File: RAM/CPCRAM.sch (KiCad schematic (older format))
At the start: 11 parts, among them J1 Conn_01x16_Female

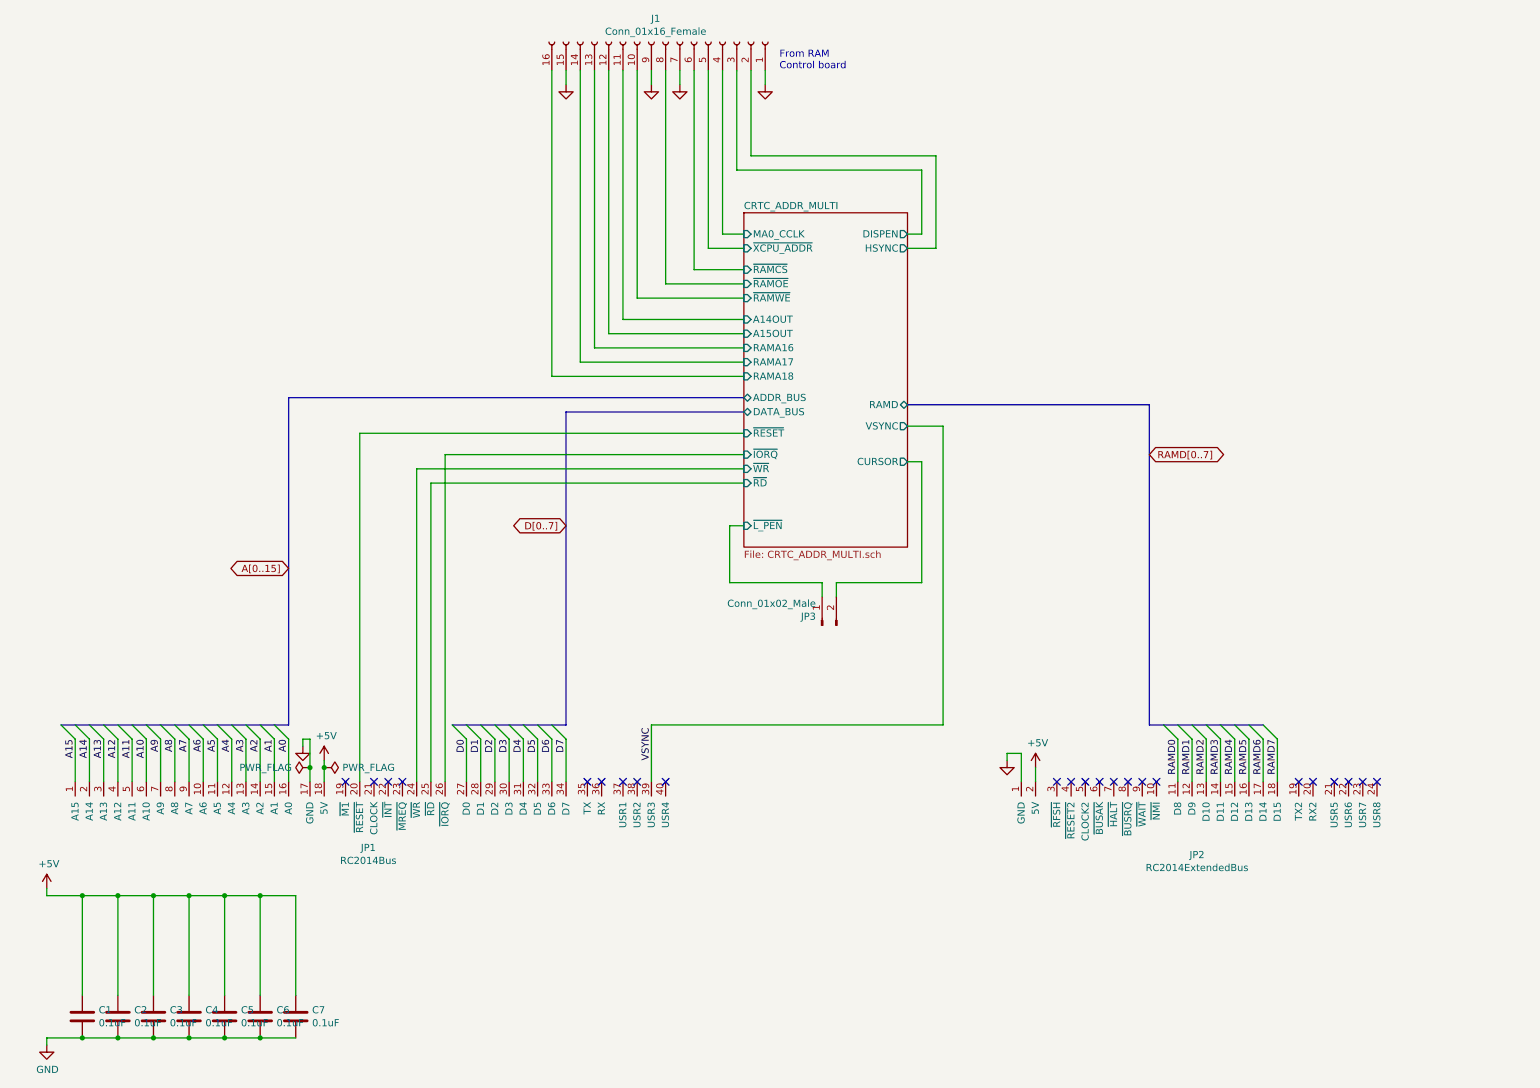
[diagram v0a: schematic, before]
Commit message: Long overdue update...
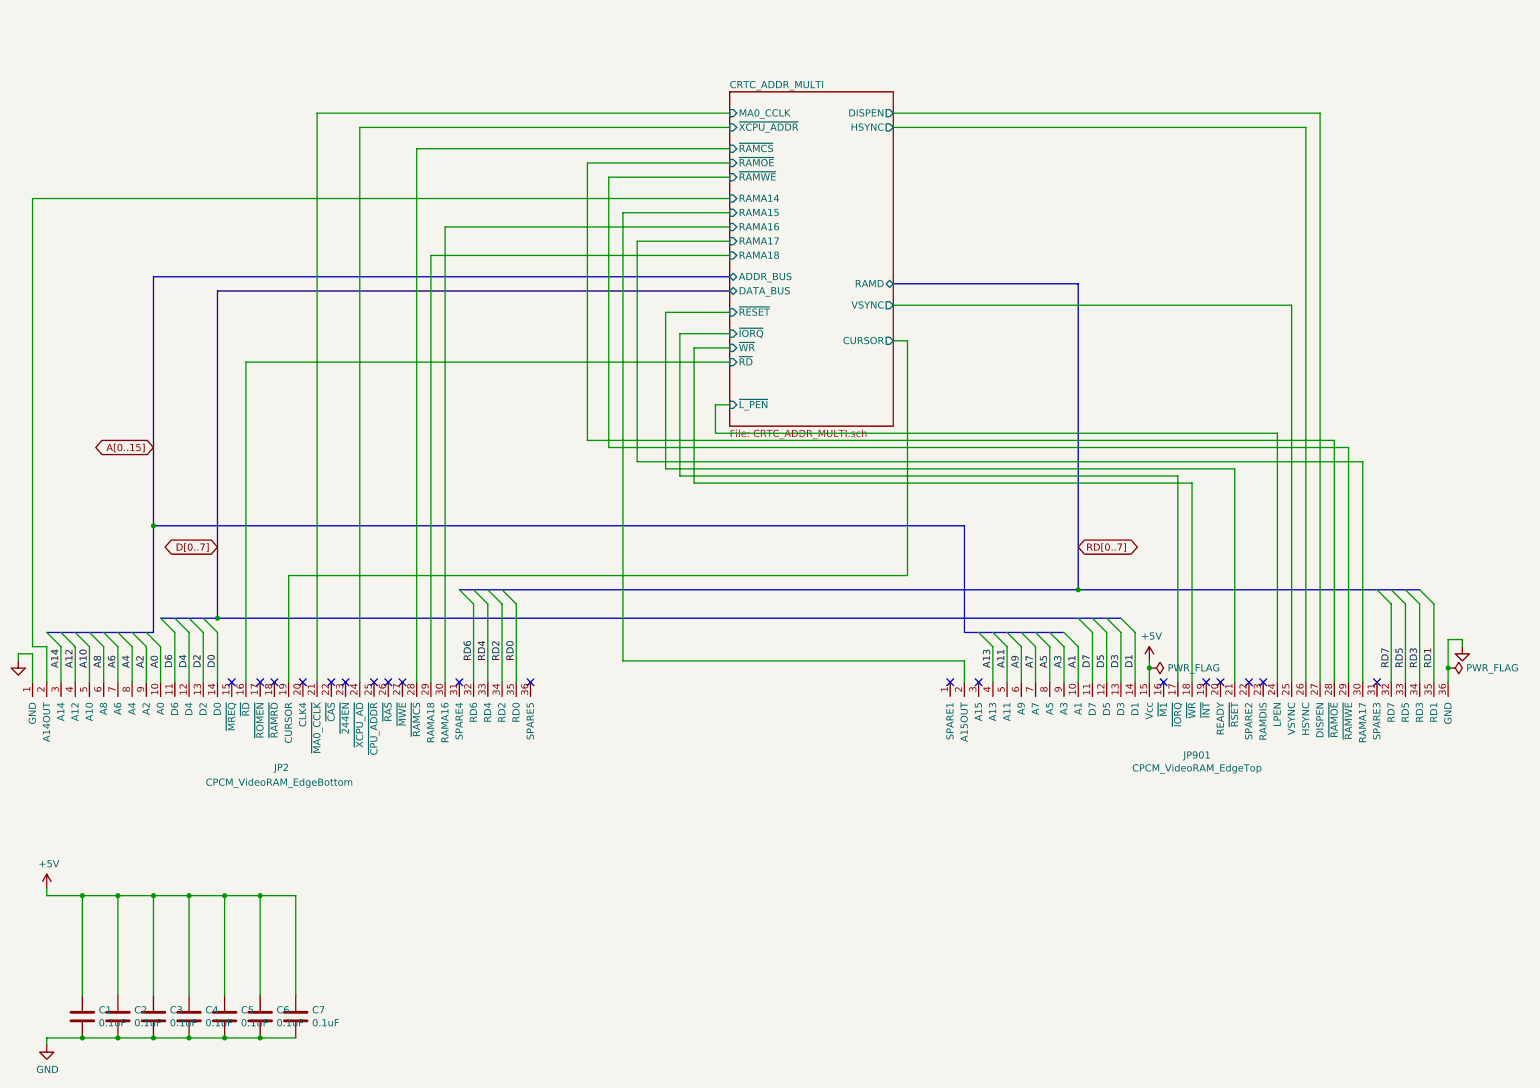
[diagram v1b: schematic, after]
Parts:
- removed J1: Conn_01x16_Female, Connector_PinSocket_2.54mm:PinSocket_2x08_P2.54mm_Vertical, symbol Connector:Conn_01x16_Female
- removed JP1: RC2014Bus, Connector_PinHeader_2.54mm:PinHeader_1x40_P2.54mm_Vertical, symbol CPCRAM-rescue:RC2014Bus-CPC
- removed JP2: RC2014ExtendedBus, Connector_PinHeader_2.54mm:PinHeader_1x25_P2.54mm_Vertical, symbol CPCRAM-rescue:RC2014ExtendedBus-CPC
- removed JP3: Conn_01x02_Male, Connector_PinHeader_2.54mm:PinHeader_1x02_P2.54mm_Vertical, symbol Connector:Conn_01x02_Male
- added JP2: CPCM_VideoRAM_EdgeBottom, CPCModular:Edge36_2.54PS, symbol CPCModular:CPCM_VideoRAM_EdgeBottom
- added JP901: CPCM_VideoRAM_EdgeTop, CPCModular:Edge36_2.54PS, symbol CPCModular:CPCM_VideoRAM_EdgeTop
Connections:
- net +5V: now also JP901.15 (Vcc)
- net A0: now also JP2.10 (A0)
- net A1: now also JP901.10 (A1)
- net A10: now also JP2.5 (A10)
- net A11: now also JP901.5 (A11)
- net A12: now also JP2.4 (A12)
- net A13: now also JP901.4 (A13)
- net A14: now also JP2.3 (A14)
- net A2: now also JP2.9 (A2)
- net A3: now also JP901.9 (A3)
- net A4: now also JP2.8 (A4)
- net A5: now also JP901.8 (A5)
- net A6: now also JP2.7 (A6)
- net A7: now also JP901.7 (A7)
- net A8: now also JP2.6 (A8)
- net A9: now also JP901.6 (A9)
- net CRTC_ADDR_MULTI/CURSOR: now also JP2.19 (CURSOR)
- net CRTC_ADDR_MULTI/DISPEN: now also JP901.27 (DISPEN)
- net CRTC_ADDR_MULTI/HSYNC: now also JP901.26 (HSYNC)
- net CRTC_ADDR_MULTI/MA0_CCLK: now also JP2.21 (~MA0_CCLK)
- net CRTC_ADDR_MULTI/RAMA16: now also JP2.30 (RAMA16)
- net CRTC_ADDR_MULTI/RAMA17: now also JP901.30 (RAMA17)
- net CRTC_ADDR_MULTI/RAMA18: now also JP2.29 (RAMA18)
- net CRTC_ADDR_MULTI/~IORQ: now also JP901.17 (~IORQ)
- net CRTC_ADDR_MULTI/~L_PEN: now also JP901.24 (LPEN)
- net CRTC_ADDR_MULTI/~RAMCS: now also JP2.28 (~RAMCS)
- net CRTC_ADDR_MULTI/~RAMOE: now also JP901.28 (~RAMOE)
- net CRTC_ADDR_MULTI/~RAMWE: now also JP901.29 (~RAMWE)
- net CRTC_ADDR_MULTI/~RD: now also JP2.16 (~RD)
- net CRTC_ADDR_MULTI/~RESET: now also JP901.21 (~RSET)
- net CRTC_ADDR_MULTI/~WR: now also JP901.18 (~WR)
- net CRTC_ADDR_MULTI/~XCPU_ADDR: now also JP2.24 (~XCPU_AD)
- net D0: now also JP2.14 (D0)
- net D1: now also JP901.14 (D1)
- net D2: now also JP2.13 (D2)
- net D3: now also JP901.13 (D3)
- net D4: now also JP2.12 (D4)
- net D5: now also JP901.12 (D5)
- net D6: now also JP2.11 (D6)
- net D7: now also JP901.11 (D7)
- net GND: now also JP2.1 (GND), JP901.36 (GND)
- new net CRTC_ADDR_MULTI/RAMA14: JP2.2 (A14OUT)
- new net CRTC_ADDR_MULTI/RAMA15: JP901.2 (A15OUT)
- new net CRTC_ADDR_MULTI/VSYNC: JP901.25 (VSYNC)
- new net RD0: JP2.35 (RD0)
- new net RD1: JP901.35 (RD1)
- new net RD2: JP2.34 (RD2)
- new net RD3: JP901.34 (RD3)
- new net RD4: JP2.33 (RD4)
- new net RD5: JP901.33 (RD5)
- new net RD6: JP2.32 (RD6)
- new net RD7: JP901.32 (RD7)
- no-connect marks 23 -> 19
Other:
- note removed: "From RAM \nControl board"
